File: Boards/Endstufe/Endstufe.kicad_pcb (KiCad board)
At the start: 2 copper layers, 153 x 111 mm, 61 parts, among them J1 HV In, J2 Relais, J3 Audio_In, J4 Übertrager, J5 Gegenkopplung, K1 G6E, P4 6V3_AC, P6 6V3_DC, P8 Bias, T1 KT88, T2 KT88, U1 ECC82, U2 ECC83

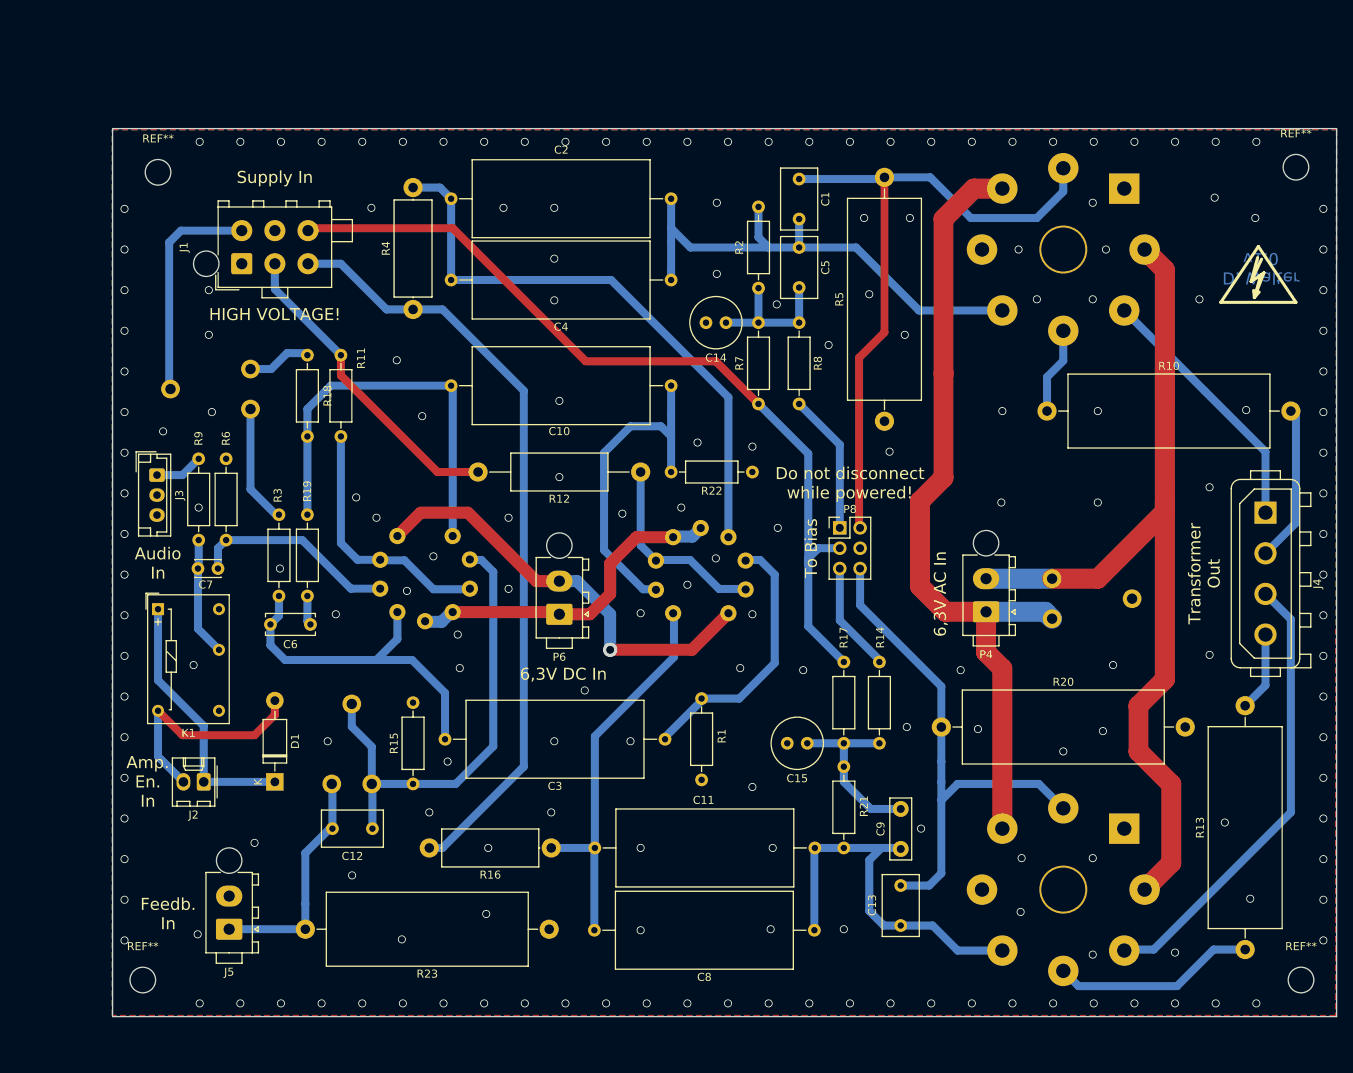
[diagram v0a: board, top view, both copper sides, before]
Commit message: Work in progess - many LAyour changes
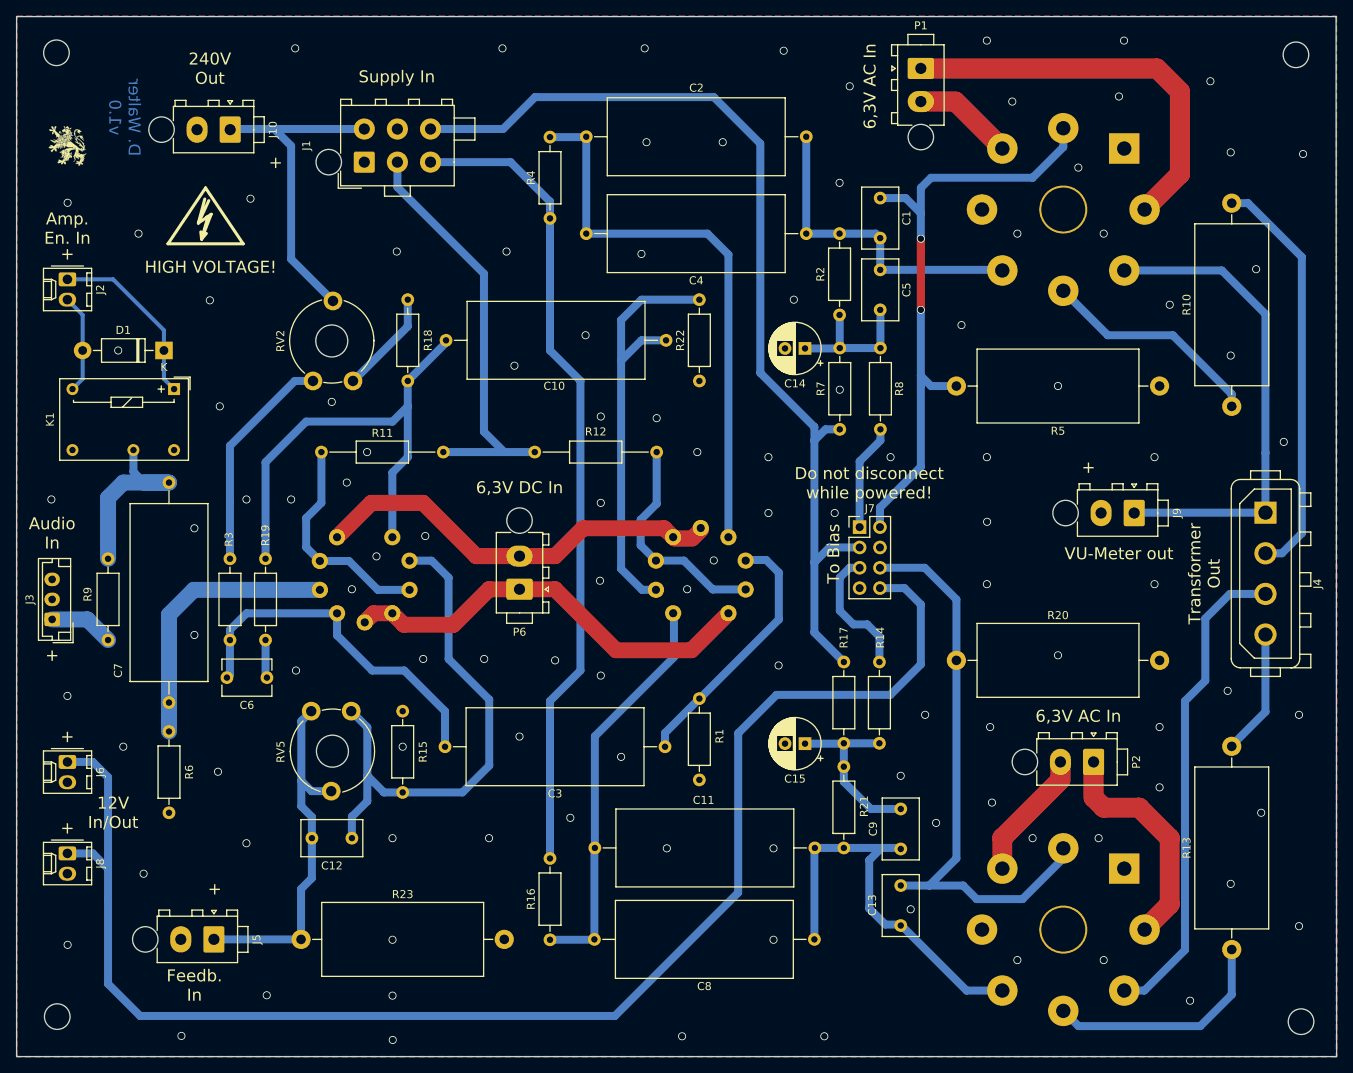
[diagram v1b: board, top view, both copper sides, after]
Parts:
- removed P4: 6V3_AC, Connector_TE-Connectivity:TE_MATE-N-LOK_1-770866-x_1x02_P4.14mm_Vertical
- removed P8: Bias, Connector_PinHeader_2.54mm:PinHeader_2x03_P2.54mm_Vertical
- removed RV3: 500R, Potentiometer_THT:Potentiometer_Piher_PT-10-V10_Vertical
- added G***: LOGO, Loewe:Loewe_Klein, F.Cu at (53.3, 53.3)
- added G***: LOGO, Loewe:Loewe_Klein, B.Cu at (66.0, 108.7)
- added J10: 240V VU, Connector_TE-Connectivity:TE_MATE-N-LOK_1-770866-x_1x02_P4.14mm_Vertical, F.Cu at (73.7, 51.3)
- added J6: 12V out, Connector_Molex:Molex_KK-254_AE-6410-02A_1x02_P2.54mm_Vertical, F.Cu at (53.3, 130.3)
- added J7: Conn_01x08, Connector_PinHeader_2.54mm:PinHeader_2x04_P2.54mm_Vertical, F.Cu at (152.3, 101.0)
- added J8: 12V In, Connector_Molex:Molex_KK-254_AE-6410-02A_1x02_P2.54mm_Vertical, F.Cu at (53.3, 141.8)
- added J9: VU-Meter, Connector_TE-Connectivity:TE_MATE-N-LOK_1-770866-x_1x02_P4.14mm_Vertical, F.Cu at (186.7, 99.2)
- added P1: 6V3_AC, Connector_TE-Connectivity:TE_MATE-N-LOK_1-770866-x_1x02_P4.14mm_Vertical, F.Cu at (160.0, 43.7)
- added P2: 6V3_AC, Connector_TE-Connectivity:TE_MATE-N-LOK_1-770866-x_1x02_P4.14mm_Vertical, F.Cu at (181.6, 130.3)
- C14, C15: value 10µF / 100V -> 10µF/100V; footprint Capacitor_THT:C_Radial_D6.3mm_H5.0mm_P2.50mm -> Capacitor_THT:CP_Radial_D6.3mm_P2.50mm
- C6: footprint Capacitor_THT:C_Disc_D6.0mm_W2.5mm_P5.00mm -> Capacitor_THT:C_Disc_D6.0mm_W4.4mm_P5.00mm
- C7: footprint Capacitor_THT:C_Disc_D3.0mm_W2.0mm_P2.50mm -> Capacitor_THT:C_Axial_L22.0mm_D9.5mm_P27.50mm_Horizontal
- C9: footprint Capacitor_THT:C_Disc_D7.5mm_W2.5mm_P5.00mm -> Capacitor_THT:C_Disc_D7.5mm_W4.4mm_P5.00mm
- R10, R13, R20, R23, R5: footprint Resistor_THT:R_Axial_Power_L25.0mm_W9.0mm_P30.48mm -> Resistor_THT:R_Axial_DIN0922_L20.0mm_D9.0mm_P25.40mm_Horizontal
- R11: value 68k -> 68k/1W; footprint Resistor_THT:R_Axial_DIN0207_L6.3mm_D2.5mm_P10.16mm_Horizontal -> Resistor_THT:R_Axial_DIN0207_L6.3mm_D2.5mm_P15.24mm_Horizontal
- R12: footprint Resistor_THT:R_Axial_DIN0414_L11.9mm_D4.5mm_P20.32mm_Horizontal -> Resistor_THT:R_Axial_DIN0207_L6.3mm_D2.5mm_P15.24mm_Horizontal
- R16, R4: footprint Resistor_THT:R_Axial_DIN0414_L11.9mm_D4.5mm_P15.24mm_Horizontal -> Resistor_THT:R_Axial_DIN0207_L6.3mm_D2.5mm_P10.16mm_Horizontal
- RV2, RV5: footprint Potentiometer_THT:Potentiometer_Piher_PT-10-V10_Vertical -> Potentiometer_THT:Potentiometer_Piher_PT-10-V10_Vertical_Hole; moved to F.Cu
- moved REF** 131.8 mm to (70.6, 62.8)
- moved J2 65.1 mm to (53.3, 70.0), turned to 270 degrees
- moved D1 55.7 mm to (65.4, 78.9), turned to 180 degrees
- moved R6 44.8 mm to (66.0, 136.7), turned to 90 degrees
- moved R5 34.7 mm to (189.8, 83.4), turned to 180 degrees
- moved K1 27.6 mm to (66.6, 83.7), turned to 270 degrees
- moved REF** 25.8 mm to (107.3, 145.6), turned to 90 degrees
- moved R9 25.3 mm to (58.4, 115.1), turned to 90 degrees
- moved R10 23.1 mm to (198.9, 85.9), turned to 90 degrees
- moved J3 22.3 mm to (51.4, 112.5), turned to 90 degrees
- moved R4 20.6 mm to (113.6, 62.4)
- moved J1 19.9 mm to (90.4, 55.4)
- moved REF** 19.6 mm to (51.9, 41.7)
- moved C2 18.6 mm to (145.7, 52.2)
- moved C4 17.9 mm to (145.7, 64.3)
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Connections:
- RV2 pad 1: Net-(R3-Pad1) -> Net-(R18-Pad2)
- RV2 pad 3: Net-(R18-Pad2) -> Net-(R3-Pad1)
- RV5 pad 2: Net-(C12-Pad1) -> Net-(C12-Pad2)
- T1 pad 2: Net-(P4-Pad2) -> Net-(P1-Pad1)
- T1 pad 7: Net-(P4-Pad1) -> Net-(P1-Pad2)
- T2 pad 2: Net-(P4-Pad2) -> Net-(P2-Pad1)
- T2 pad 7: Net-(P4-Pad1) -> Net-(P2-Pad2)
- U1 pad 4: Net-(P6-Pad1) -> Net-(P6-Pad2)
- U1 pad 5: Net-(P6-Pad1) -> Net-(P6-Pad2)
- U1 pad 9: Net-(P6-Pad2) -> Net-(P6-Pad1)
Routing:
- net +12V: track 0.00 -> 184.2 mm
- net Net-(P4-Pad2): track 116.4 -> 0.00 mm
- net Net-(P4-Pad1): track 102.2 -> 0.00 mm
- net Net-(P1-Pad1): track 0.00 -> 50.2 mm
- net Net-(J4-Pad2): track 19.6 -> 51.7 mm
- net Net-(P2-Pad1): track 0.00 -> 28.8 mm
- net /+450V_T1: track 32.7 -> 61.2 mm
- net Net-(C1-Pad2): track 65.0 -> 40.9 mm
- net -60V: track 107.5 -> 124.6 mm
- net Net-(R10-Pad1): track 10.9 -> 28.0 mm
- net Net-(D1-Pad2): track 28.9 -> 12.5 mm
- net Net-(P2-Pad2): track 0.00 -> 16.3 mm
- net Net-(C12-Pad2): track 29.3 -> 45.5 mm
- net -120V: track 39.5 -> 53.2 mm
- net +240V: track 28.1 -> 41.3 mm
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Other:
- board size 153 x 111 mm -> 165 x 130 mm
- board text added: "+"
- board text added: "12V In/Out"
- board text added: "240V Out"
- board text added: "Driver Sym. Adjust"
- board text added: "HIGH VOLTAGE! Do not Touch Board when powered!"
- board text added: "VU-Meter out"
- board text removed: "Driver Bias Adjust"
- board text removed: "KT88 Heater Adjust"
